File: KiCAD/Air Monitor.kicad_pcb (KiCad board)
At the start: 2 copper layers, 50.1 x 52.7 mm, 16 parts, among them J1 Barrel_Jack, U1 ESP32-DevKitC, U2 BME680, U3 SGP40

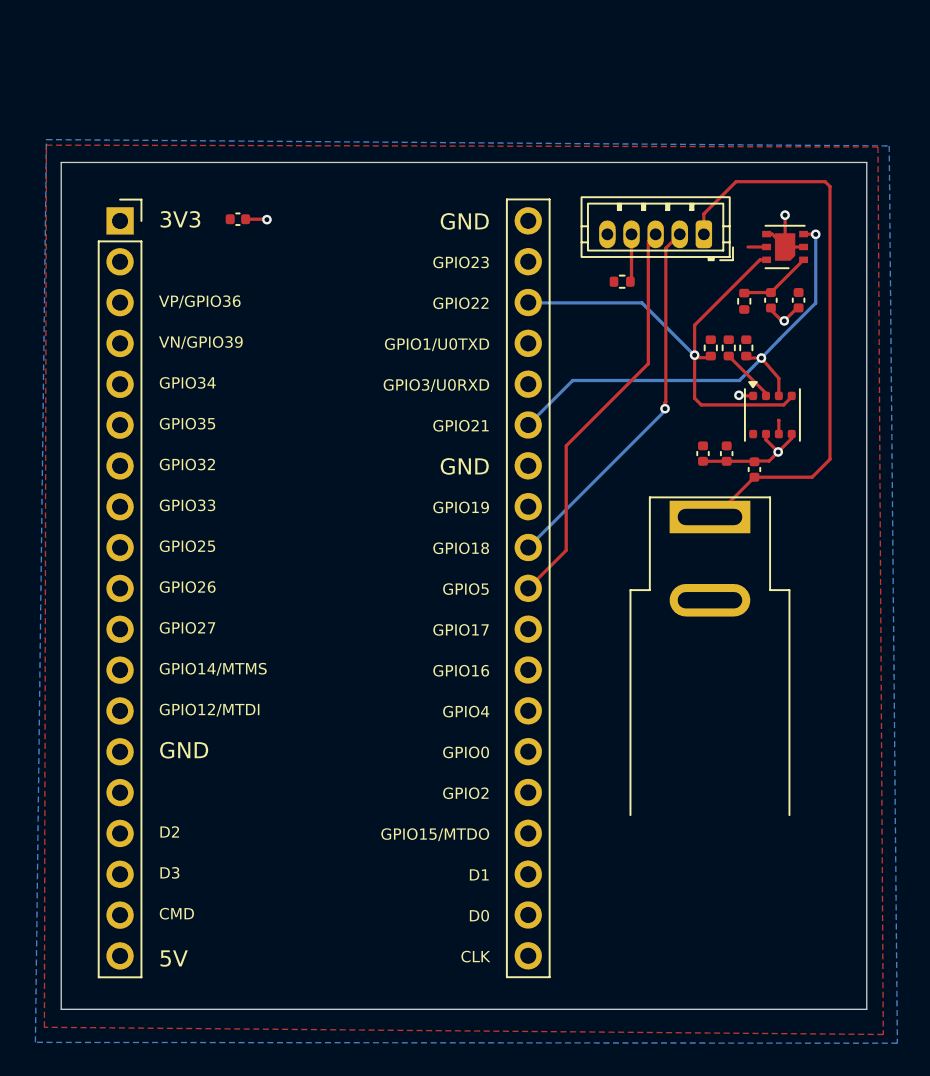
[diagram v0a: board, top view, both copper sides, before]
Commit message: PCB updates
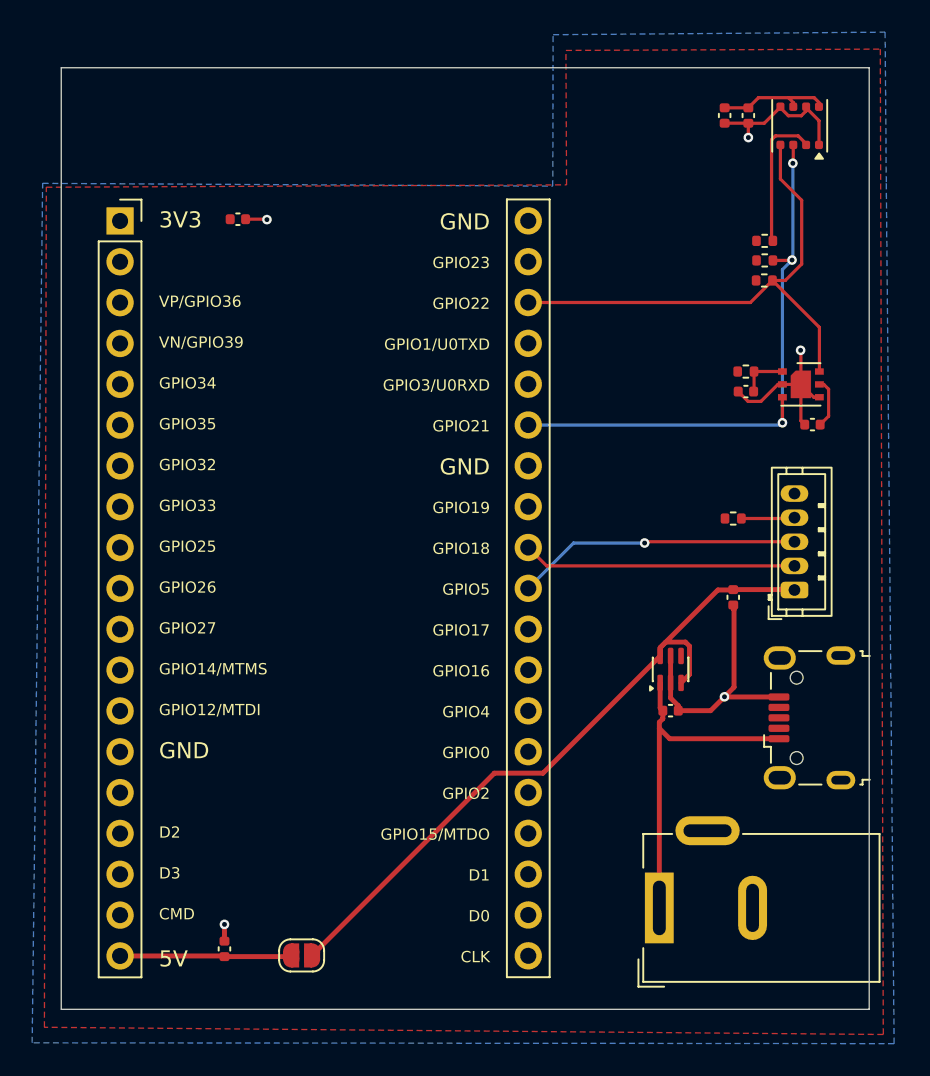
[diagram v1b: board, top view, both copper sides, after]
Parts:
- added C7: 10μF, Capacitor_SMD:C_0402_1005Metric, F.Cu at (189.9, 116.8)
- added C8: 1μF, Capacitor_SMD:C_0402_1005Metric, F.Cu at (186.0, 123.9)
- added J2: USB_B_Micro, Connector_USB:USB_Micro-B_Wuerth_629105150521, F.Cu at (194.6, 124.3)
- added JP1: SolderJumper_2_Open, Jumper:SolderJumper-2_P1.3mm_Open_RoundedPad1.0x1.5mm, F.Cu at (163.0, 139.1)
- added U4: LM66100DCK, Package_TO_SOT_SMD:SOT-363_SC-70-6, F.Cu at (186.0, 121.3)
- J1: footprint Connector_BarrelJack:BarrelJack_SwitchcraftConxall_RAPC10U_Horizontal -> Connector_BarrelJack:BarrelJack_Wuerth_6941xx301002
- moved C2 44.5 mm to (158.2, 138.7)
- moved J1 24.5 mm to (185.3, 136.1)
- moved SPS30 22.8 mm to (193.7, 116.4), turned to 90 degrees
- moved C4 21.1 mm to (189.4, 86.8)
- moved C3 21.1 mm to (190.8, 86.8)
- moved U2 18.1 mm to (194.0, 87.5), turned to 180 degrees
- moved R4 16.3 mm to (189.9, 111.9)
- moved U3 8.60 mm to (194.1, 103.6), turned to 0 degrees
- moved C5 7.78 mm to (194.8, 106.1), turned to 180 degrees
- moved R3 7.02 mm to (191.8, 94.6), turned to 180 degrees
- moved C6 5.89 mm to (190.7, 104.0), turned to 180 degrees
- moved R2 5.56 mm to (191.8, 95.9), turned to 180 degrees
- moved R1 5.35 mm to (191.8, 97.1), turned to 180 degrees
- moved R5 4.37 mm to (190.7, 102.8), turned to 180 degrees
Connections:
- net Net-(U3-VDD) renamed /SGP VDD
- C2 pad 2: +5V -> /ESP 5V Pin
- J1 pad 1: +5V -> 5V INPUT
- U1 pad 19: unconnected-(U1-5V-Pad19) -> /ESP 5V Pin
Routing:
- net 5V INPUT: track 0.00 -> 22.2 mm
- net GND: track 17.9 -> 39.4 mm
- net /ESP 5V Pin: track 0.00 -> 10.9 mm
- net +5V: track 36.1 -> 44.4 mm
- net +3.3V: track 2.05 -> 10.3 mm
- net /RX: track 25.3 -> 17.7 mm, vias 0 -> 1
- net /SDA: track 29.9 -> 36.4 mm, vias 2 -> 3
- net /TX: track 23.4 -> 17.0 mm, vias 1 -> 0
- net /CS: track 3.44 -> 8.84 mm
- net /SCL: track 30.0 -> 32.9 mm, vias 1 -> 0
- net /SGP VDD: track 4.55 -> 3.02 mm
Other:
- board size 50.1 x 52.7 mm -> 50.3 x 58.6 mm
